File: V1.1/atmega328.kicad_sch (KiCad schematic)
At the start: 25 parts, among them J1 Conn_01x04, J2 Conn_01x02, J3 Conn_01x02_Male, J4 Conn_01x03, J5 Conn_01x08, Q1 Si2319CDS, U1 ATmega328P-AU, U2 AS5048A, Y1 Crystal

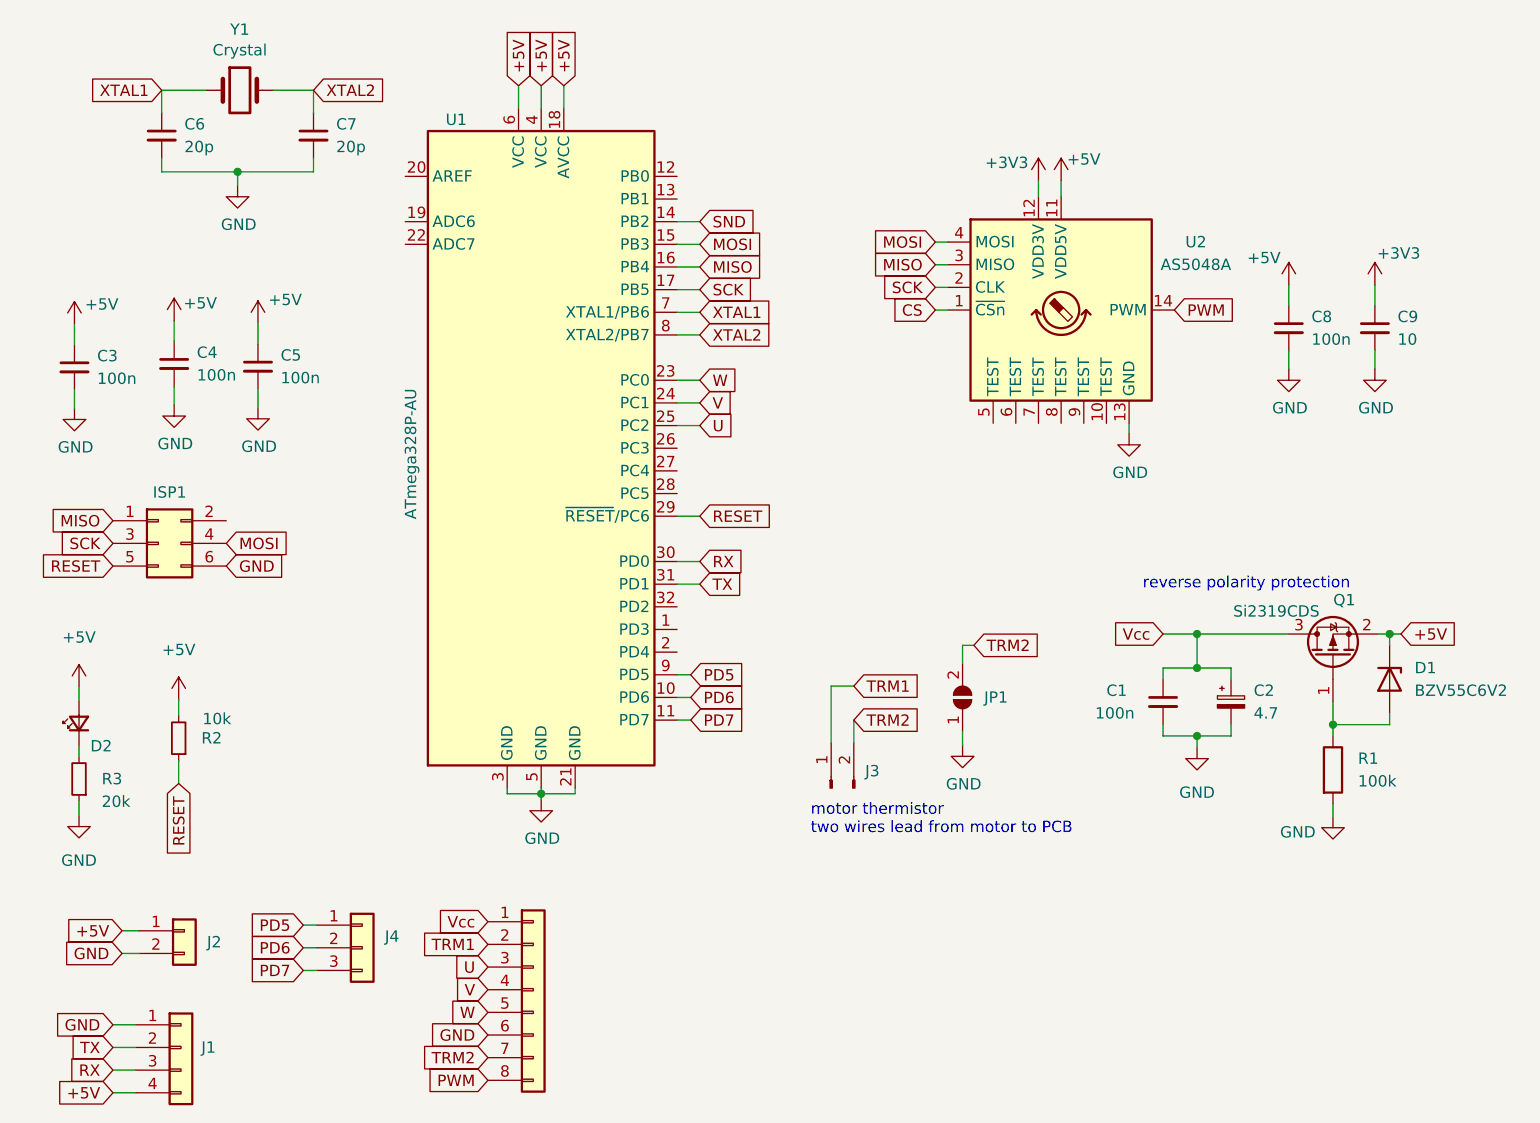
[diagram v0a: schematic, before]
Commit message: JCLPCB V1.2 order
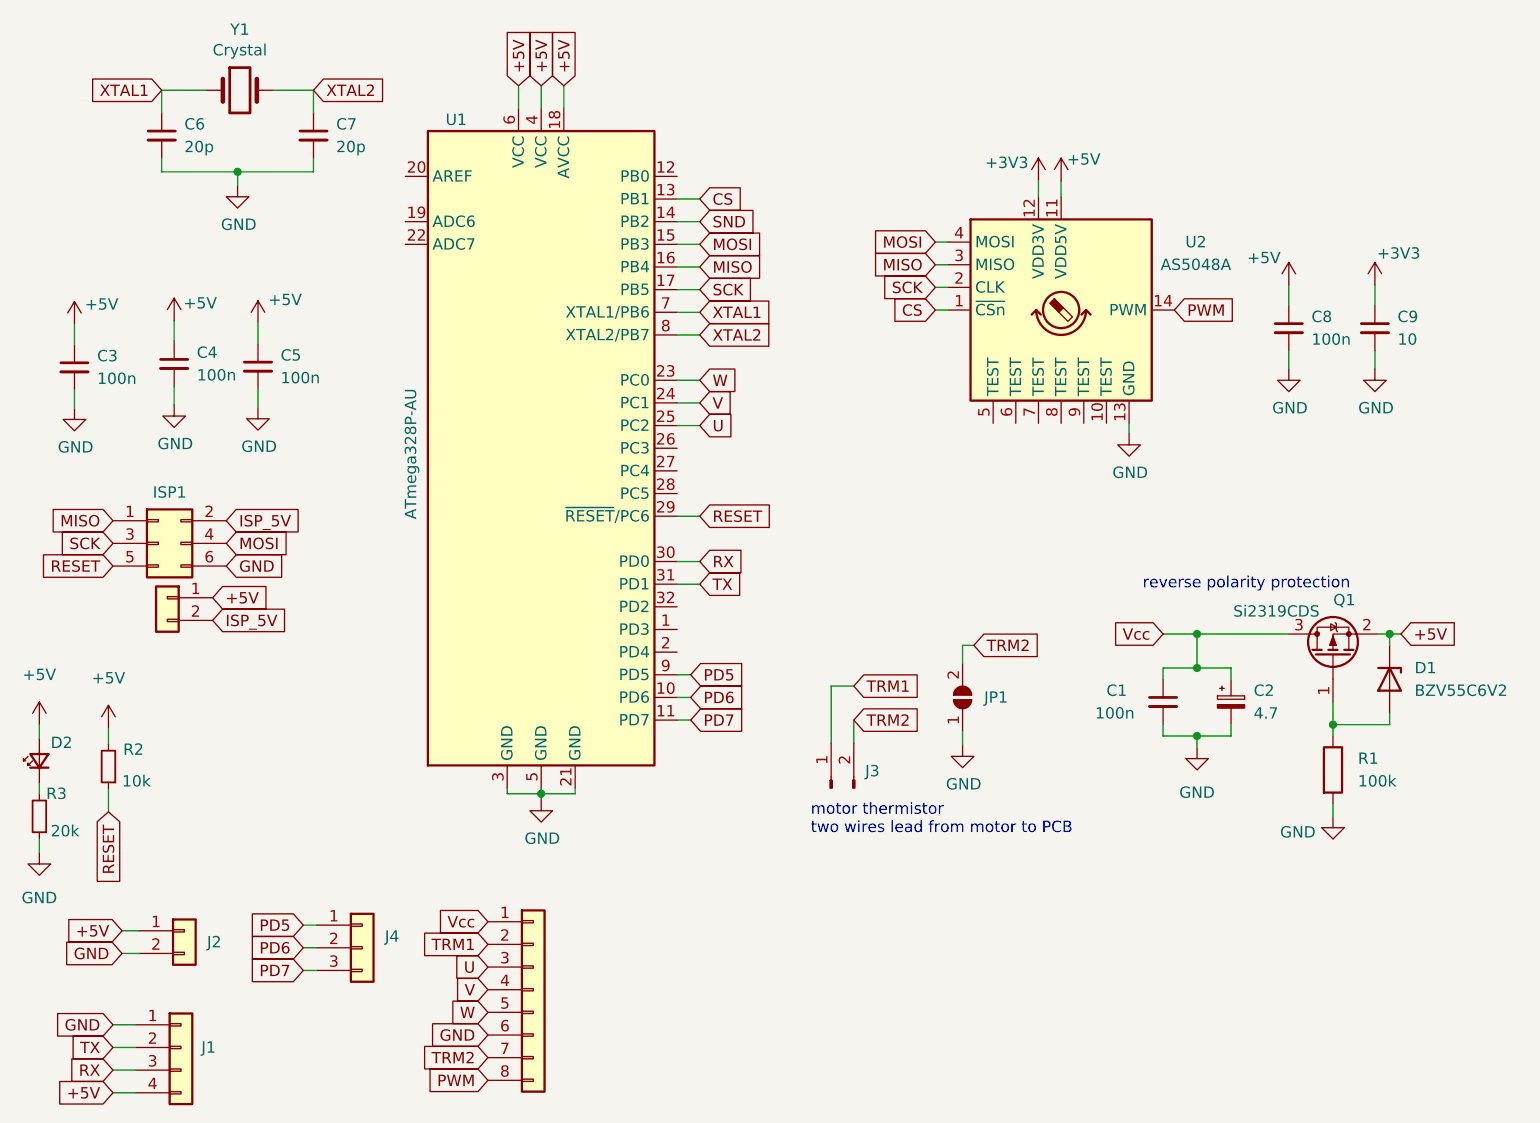
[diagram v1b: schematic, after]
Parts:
- added J6: Conn_01x02, Connector_PinHeader_2.54mm:PinHeader_1x02_P2.54mm_Vertical, symbol Connector_Generic:Conn_01x02
- C6, C7: LCSC C880615 -> C76959
- C9: LCSC C1525 -> C315248
- ISP1, J1, J2, J4, J5, JP1: now left out of the parts list
- U1: LCSC (none) -> C14877
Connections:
- net +5V: now also J6.1 (Pin_1)
- net CS: now also U1.13 (PB1)
- net ISP_5V: now reaches ISP1.2 (Pin_2)
- net ISP_5V: now also J6.2 (Pin_2)
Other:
- moved on the sheet: D2, R2, R3
